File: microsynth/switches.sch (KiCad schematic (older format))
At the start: 35 parts, among them SW12 SOURCE, SW13 THUMBWEEL, SW14 SW_SPDT, SW15 SW_SPDT, SW16 SW_SPDT, SW17 SW_SPDT, SW2 RANGE, SW21 SW_Rotary2x6, SW3 SW_DPTT_SELECTOR, SW4 SW_DPTT_SELECTOR, SW5 SW_SPDT, SW6 SW_DPTT_SELECTOR, U22 4013, U7 LM741

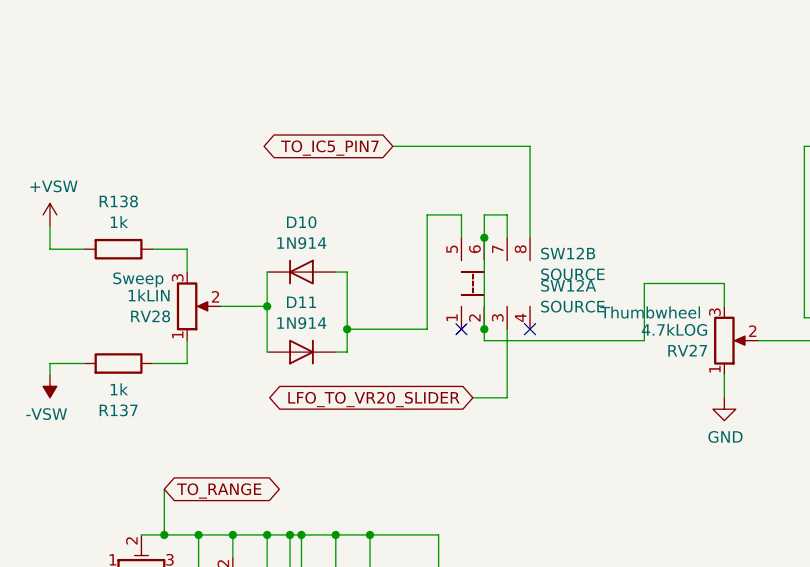
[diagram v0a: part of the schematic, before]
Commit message: Layout...
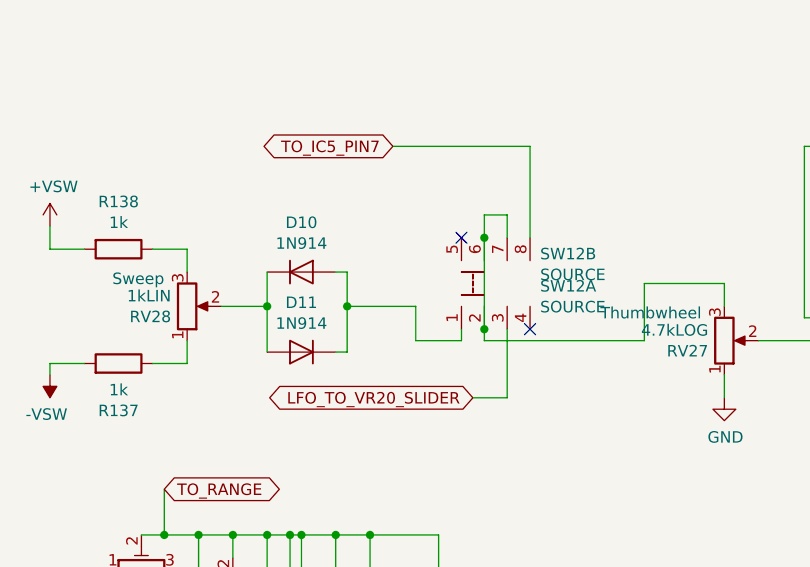
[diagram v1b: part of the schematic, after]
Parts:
- SW12, SW13, SW3: footprint Buttons_Switches_ThroughHole:DP3T_Toggle -> Buttons_Switches_ThroughHole:L203011MS02Q
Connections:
- net at D10.2 (A), D11.1 (K): now also SW12.1; no longer SW12.5
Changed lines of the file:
@@
 F 0 "SW3" H 7594 1338 50  0000 L CNN
 F 1 "SW_DPTT_SELECTOR" H 7594 1247 50  0000 L CNN
-F 2 "Buttons_Switches_ThroughHole:DP3T_Toggle" H 7400 1350 50  0001 C CNN
+F 2 "Buttons_Switches_ThroughHole:L203011MS02Q" H 7400 1350 50  0001 C CNN
 F 3 "" H 7400 1350 50  0001 C CNN
 	1    7400 1350
@@
 F 0 "SW3" H 7594 1379 50  0000 L CNN
 F 1 "SW_DPTT_SELECTOR" H 7594 1288 50  0000 L CNN
-F 2 "Buttons_Switches_ThroughHole:DP3T_Toggle" H 7400 1250 50  0001 C CNN
+F 2 "Buttons_Switches_ThroughHole:L203011MS02Q" H 7400 1250 50  0001 C CNN
 F 3 "" H 7400 1250 50  0001 C CNN
 	2    7400 1250
@@
 F 0 "SW12" H 5594 4488 50  0000 L CNN
 F 1 "SOURCE" H 5594 4397 50  0000 L CNN
-F 2 "Buttons_Switches_ThroughHole:DP3T_Toggle" H 5400 4500 50  0001 C CNN
+F 2 "Buttons_Switches_ThroughHole:L203011MS02Q" H 5400 4500 50  0001 C CNN
 F 3 "" H 5400 4500 50  0001 C CNN
 	1    5400 4500
@@
 F 0 "SW12" H 5594 4629 50  0000 L CNN
 F 1 "SOURCE" H 5594 4538 50  0000 L CNN
-F 2 "Buttons_Switches_ThroughHole:DP3T_Toggle" H 5400 4500 50  0001 C CNN
+F 2 "Buttons_Switches_ThroughHole:L203011MS02Q" H 5400 4500 50  0001 C CNN
 F 3 "" H 5400 4500 50  0001 C CNN
 	2    5400 4500
 	1    0    0    -1
 $EndComp
-Connection ~ 4750 4700
-Wire Wire Line
-	4750 4700 4750 4800
 Wire Wire Line
 	5350 4700 5350 4750
@@
 F 0 "SW13" H 7394 4438 50  0000 L CNN
 F 1 "THUMBWEEL" H 7394 4347 50  0000 L CNN
-F 2 "Buttons_Switches_ThroughHole:DP3T_Toggle" H 7200 4450 50  0001 C CNN
+F 2 "Buttons_Switches_ThroughHole:L203011MS02Q" H 7200 4450 50  0001 C CNN
 F 3 "" H 7200 4450 50  0001 C CNN
 	1    7200 4450
@@
 F 0 "SW13" H 7394 4579 50  0000 L CNN
 F 1 "THUMBWEEL" H 7394 4488 50  0000 L CNN
-F 2 "Buttons_Switches_ThroughHole:DP3T_Toggle" H 7200 4450 50  0001 C CNN
+F 2 "Buttons_Switches_ThroughHole:L203011MS02Q" H 7200 4450 50  0001 C CNN
 F 3 "" H 7200 4450 50  0001 C CNN
 	2    7200 4450
@@
 	3250 650  3250 850
 Connection ~ 3250 850
-Wire Wire Line
-	4750 4450 4750 4700
 Text GLabel 1200 900  2    50   BiDi ~ 0
 TO_VR20_SLIDER_VCO2_OUTPUT
@@
 Connection ~ 5350 4300
 Wire Wire Line
-	5100 4700 5100 4200
-Wire Wire Line
-	5100 4200 5250 4200
-Wire Wire Line
-	5250 4200 5250 4300
-Wire Wire Line
-	5100 4700 4750 4700
-Wire Wire Line
 	5150 6150 5150 6900
 Wire Wire Line
@@
 Wire Wire Line
 	2950 6300 3650 6300
-NoConn ~ 5250 4700
 Wire Wire Line
 	7150 4250 7150 4650
@@
 TO_KBD_R141
 NoConn ~ 3800 950
+Wire Wire Line
+	4750 4450 4750 4600
+NoConn ~ 5250 4300
+Wire Wire Line
+	5250 4700 5250 4750
+Wire Wire Line
+	5250 4750 5050 4750
+Wire Wire Line
+	5050 4750 5050 4600
+Wire Wire Line
+	5050 4600 4750 4600
+Connection ~ 4750 4600
+Wire Wire Line
+	4750 4600 4750 4800
 $EndSCHEMATC
